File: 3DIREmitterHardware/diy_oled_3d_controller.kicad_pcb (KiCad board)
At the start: 2 copper layers, 37.5 x 59.1 mm, 20 parts, among them Q1 AO3400A, U1 OPT101P, U2 OPT101P

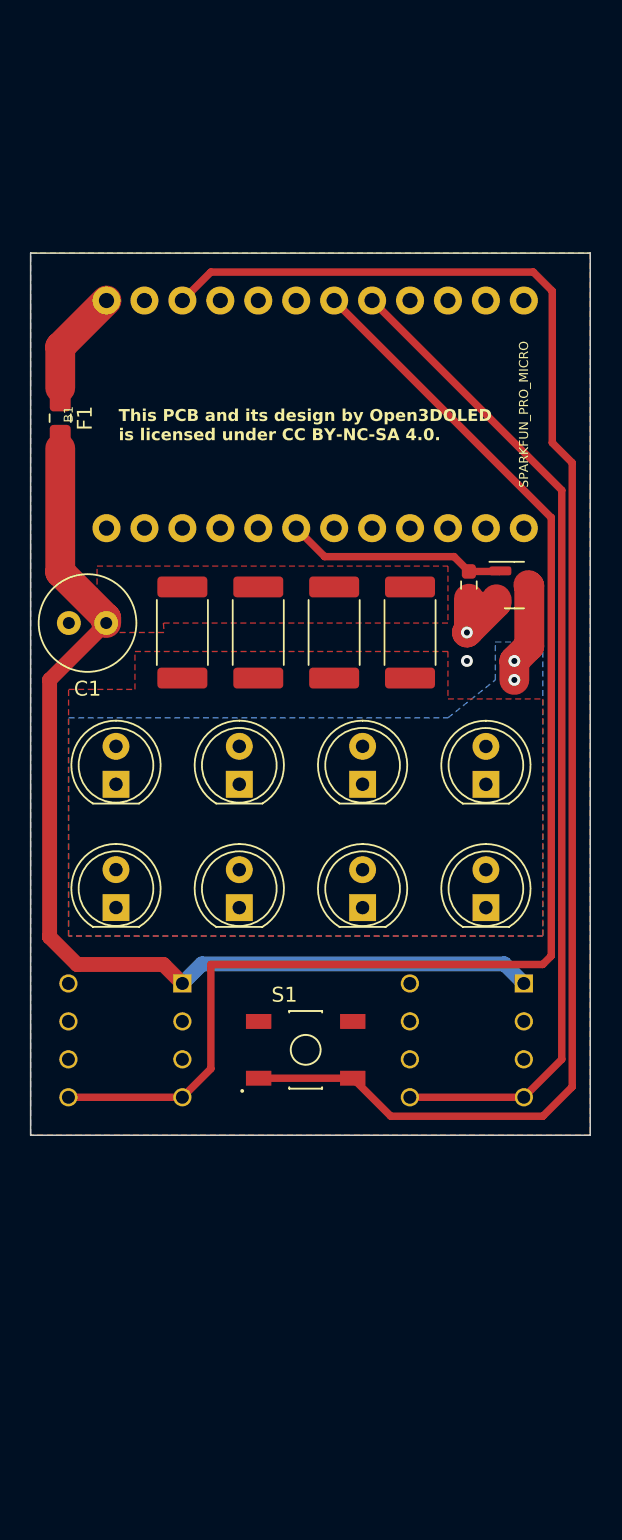
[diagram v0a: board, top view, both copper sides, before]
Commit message: initial v2 pcb hardware design
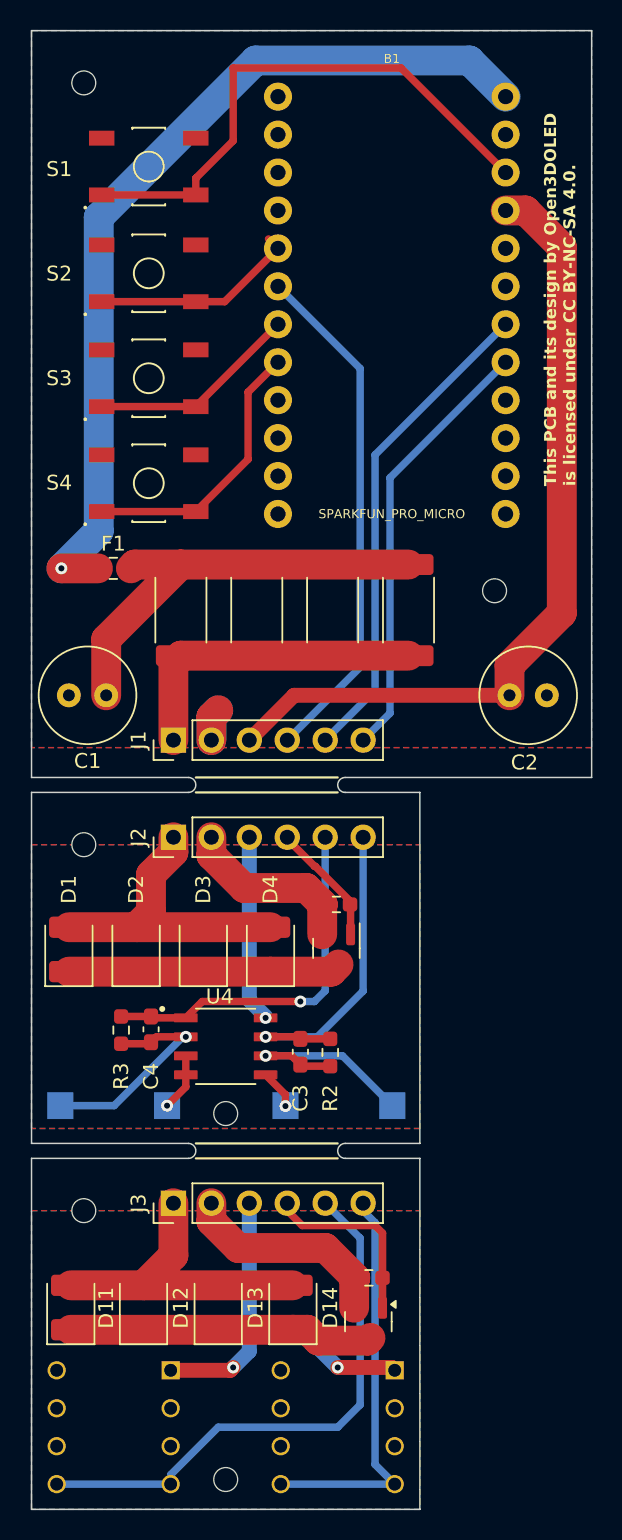
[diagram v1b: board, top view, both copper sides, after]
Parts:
- removed D5, D6, D7, D8: LED, LED_THT:LED_D5.0mm
- added C2: C_Polarized, Capacitor_THT:C_Radial_D6.3mm_H11.0mm_P2.50mm, F.Cu at (123.5, 78.5)
- added C3: 100nF, Capacitor_SMD:C_0603_1608Metric_Pad1.08x0.95mm_HandSolder, F.Cu at (109.5, 102.4)
- added C4: 100nF, Capacitor_SMD:C_0603_1608Metric_Pad1.08x0.95mm_HandSolder, F.Cu at (99.5, 100.9)
- added D10: VBPW34S, VBPW34S:XDCR_VBPW34S, B.Cu at (97.0, 106.0)
- added D11: LED, LED_SMD:LED_1210_3225Metric_Pad1.42x2.65mm_HandSolder, F.Cu at (94.1, 119.5)
- added D12: LED, LED_SMD:LED_1210_3225Metric_Pad1.42x2.65mm_HandSolder, F.Cu at (99.0, 119.5)
- added D13: LED, LED_SMD:LED_1210_3225Metric_Pad1.42x2.65mm_HandSolder, F.Cu at (104.0, 119.5)
- added D14: LED, LED_SMD:LED_1210_3225Metric_Pad1.42x2.65mm_HandSolder, F.Cu at (109.0, 119.5)
- added D9: VBPW34S, VBPW34S:XDCR_VBPW34S, B.Cu at (112.1, 106.0)
- added H1: MountingHole, Library:MountingHole_1.6mm_M1.4_ISO7380, F.Cu at (95.0, 37.5)
- added H2: MountingHole, Library:MountingHole_1.6mm_M1.4_ISO7380, F.Cu at (122.5, 71.5)
- added H3: MountingHole, Library:MountingHole_1.6mm_M1.4_ISO7380, F.Cu at (95.0, 88.5)
- added H4: MountingHole, Library:MountingHole_1.6mm_M1.4_ISO7380, F.Cu at (104.5, 106.5)
- added H5: MountingHole, Library:MountingHole_1.6mm_M1.4_ISO7380, F.Cu at (95.0, 113.0)
- added H6: MountingHole, Library:MountingHole_1.6mm_M1.4_ISO7380, F.Cu at (104.5, 131.0)
- added J1: Conn_01x06_Pin, Connector_PinHeader_2.54mm:PinHeader_1x06_P2.54mm_Vertical, F.Cu at (101.0, 81.5)
- added J2: Conn_01x06_Pin, Connector_PinHeader_2.54mm:PinHeader_1x06_P2.54mm_Vertical, F.Cu at (101.0, 88.0)
- added J3: Conn_01x06_Pin, Connector_PinHeader_2.54mm:PinHeader_1x06_P2.54mm_Vertical, F.Cu at (101.0, 112.5)
- added Q2: AO3400A, Package_TO_SOT_SMD:SOT-23, F.Cu at (114.0, 120.4)
- added R2: 10k, Resistor_SMD:R_0603_1608Metric_Pad0.98x0.95mm_HandSolder, F.Cu at (111.5, 102.4)
- added R3: 10k, Resistor_SMD:R_0603_1608Metric_Pad0.98x0.95mm_HandSolder, F.Cu at (97.5, 100.9)
- added R4: 1000, Resistor_SMD:R_0603_1608Metric_Pad0.98x0.95mm_HandSolder, F.Cu at (114.1, 117.5)
- added S2: TL3342F160QG, Tactile.Switch:SW_TL3342F160QG, F.Cu at (99.3, 50.2)
- added S3: TL3342F160QG, Tactile.Switch:SW_TL3342F160QG, F.Cu at (99.3, 57.3)
- added S4: TL3342F160QG, Tactile.Switch:SW_TL3342F160QG, F.Cu at (99.3, 64.3)
- added U4: MCP6022-I_SN, MCP6022-I_SN:SOIC127P599X175-8N, F.Cu at (104.5, 102.0)
- D1, D2, D3, D4: footprint LED_THT:LED_D5.0mm -> LED_SMD:LED_1210_3225Metric_Pad1.42x2.65mm_HandSolder
- moved S1 60.1 mm to (99.3, 43.1)
- moved U2 27.3 mm to (112.0, 127.5)
- moved Q1 27.1 mm to (111.9, 95.4), turned to -90 degrees
- moved U1 25.9 mm to (97.0, 127.5)
- moved R1 23.1 mm to (111.9, 92.5), turned to 180 degrees
- moved D4 18.2 mm to (107.5, 95.5)
- moved D3 15.4 mm to (103.0, 95.5)
- moved D2 13.0 mm to (98.5, 95.5)
- moved D1 11.5 mm to (94.0, 95.5)
- moved B1 10.7 mm to (115.6, 51.1), turned to 0 degrees
- moved F1 10.7 mm to (97.0, 70.0), turned to 0 degrees
- moved C1 4.84 mm to (96.5, 78.5)
- moved R10 1.50 mm to (116.7, 72.8)
- moved R11 1.50 mm to (111.7, 72.8)
- moved R12 1.50 mm to (106.6, 72.8)
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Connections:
- net +5V renamed +5V_1
- net /LED_MOSFET renamed /LED_MOSFET_2
- B1 pad 17: /RIGHT_OPT101_OUTPUT -> /RIGHT_SIGNAL_1
- B1 pad 18: /LEFT_OPT101_OUTPUT -> /LEFT_SIGNAL_1
- B1 pad 21: unconnected-(B1-VCC-Pad21) -> /VCC_1
- B1 pad 23: GND -> GND1
- B1 pad 5: unconnected-(B1-2-Pad5) -> Net-(B1-2)
- B1 pad 6: /LED_CONTROL -> /LED_CONTROL_1
- B1 pad 7: unconnected-(B1-4-Pad7) -> Net-(B1-4)
- B1 pad 8: unconnected-(B1-*5-Pad8) -> Net-(B1-*5)
- C1 pad 2: GND -> GND1
- D1 pad 2: /RESISTOR_LED -> /LED_POWER_2
- D2 pad 2: /RESISTOR_LED -> /LED_POWER_2
- D3 pad 2: /RESISTOR_LED -> /LED_POWER_2
- D4 pad 2: /RESISTOR_LED -> /LED_POWER_2
- Q1 pad 1: /LED_CONTROL -> /LED_CONTROL_2
- Q1 pad 2: GND -> GND2
- R1 pad 1: /LED_CONTROL -> /LED_CONTROL_2
- R1 pad 2: GND -> GND2
- R10 pad 2: /RESISTOR_LED -> /LED_POWER_1
- R11 pad 2: /RESISTOR_LED -> /LED_POWER_1
- R12 pad 2: /RESISTOR_LED -> /LED_POWER_1
- R13 pad 2: /RESISTOR_LED -> /LED_POWER_1
- S1 pad 3: GND -> GND1
- S1 pad 4: GND -> GND1
- U1 pad 1: /5V_AFTER_FUSE -> /VCC_3
- U1 pad 3: GND -> GND3
- U1 pad 4: /LEFT_OPT101_OUTPUT -> /LEFT_SIGNAL_3
- U1 pad 5: /LEFT_OPT101_OUTPUT -> /LEFT_SIGNAL_3
- U1 pad 8: GND -> GND3
- U2 pad 1: /5V_AFTER_FUSE -> /VCC_3
- U2 pad 3: GND -> GND3
- U2 pad 4: /RIGHT_OPT101_OUTPUT -> /RIGHT_SIGNAL_3
- U2 pad 5: /RIGHT_OPT101_OUTPUT -> /RIGHT_SIGNAL_3
- U2 pad 8: GND -> GND3
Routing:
- net /LEFT_OPT101_OUTPUT: track 90.2 -> 0.00 mm
- net /RIGHT_OPT101_OUTPUT: track 67.3 -> 0.00 mm
- net Net-(B1-RESET): track 102.8 -> 37.0 mm
- net /VCC_1: track 0.00 -> 54.9 mm
- net +5V_1: track 7.13 -> 59.6 mm, vias 0 -> 1
- net /5V_AFTER_FUSE: track 69.7 -> 29.5 mm
- net /LEFT_SIGNAL_3: track 0.00 -> 37.3 mm
- net /LED_CONTROL_1: track 0.00 -> 34.7 mm
- net /LEFT_SIGNAL_1: track 0.00 -> 32.8 mm
- net /RIGHT_SIGNAL_1: track 0.00 -> 29.3 mm
- net /RIGHT_SIGNAL_3: track 0.00 -> 27.3 mm
- net /VCC_3: track 0.00 -> 26.6 mm, vias 0 -> 2
- net /LEFT_SIGNAL_2: track 0.00 -> 24.7 mm, vias 0 -> 1
- net /RIGHT_SIGNAL_2: track 0.00 -> 22.5 mm, vias 0 -> 1
- net /LED_POWER_3: track 0.00 -> 21.2 mm
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- added copper zone on B.Cu, net GND1
- added copper zone on F.Cu, net GND1
- added copper zone on B.Cu, net GND2
- added copper zone on F.Cu, net GND2
- added copper zone on B.Cu, net GND3
- added copper zone on F.Cu, net GND3
- removed copper zone on F.Cu, net /5V_AFTER_FUSE
- removed copper zone on B.Cu, net /LED_MOSFET_2
- removed copper zone on F.Cu, net /RESISTOR_LED
- removed copper zone on B.Cu, net GND
- removed copper zone on F.Cu, net GND
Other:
- board size 37.5 x 59.1 mm -> 37.5 x 99 mm
